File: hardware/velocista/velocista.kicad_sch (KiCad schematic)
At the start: 15 parts, among them J1 XT30, J2 Cable_PAD, J3 Cable_PAD, J4 QTR8a, SW1 SW_Push, SW3 SW_SPDT, U1 TB6612FNG, U2 Mini360, U3 ESP32_DEVKITC

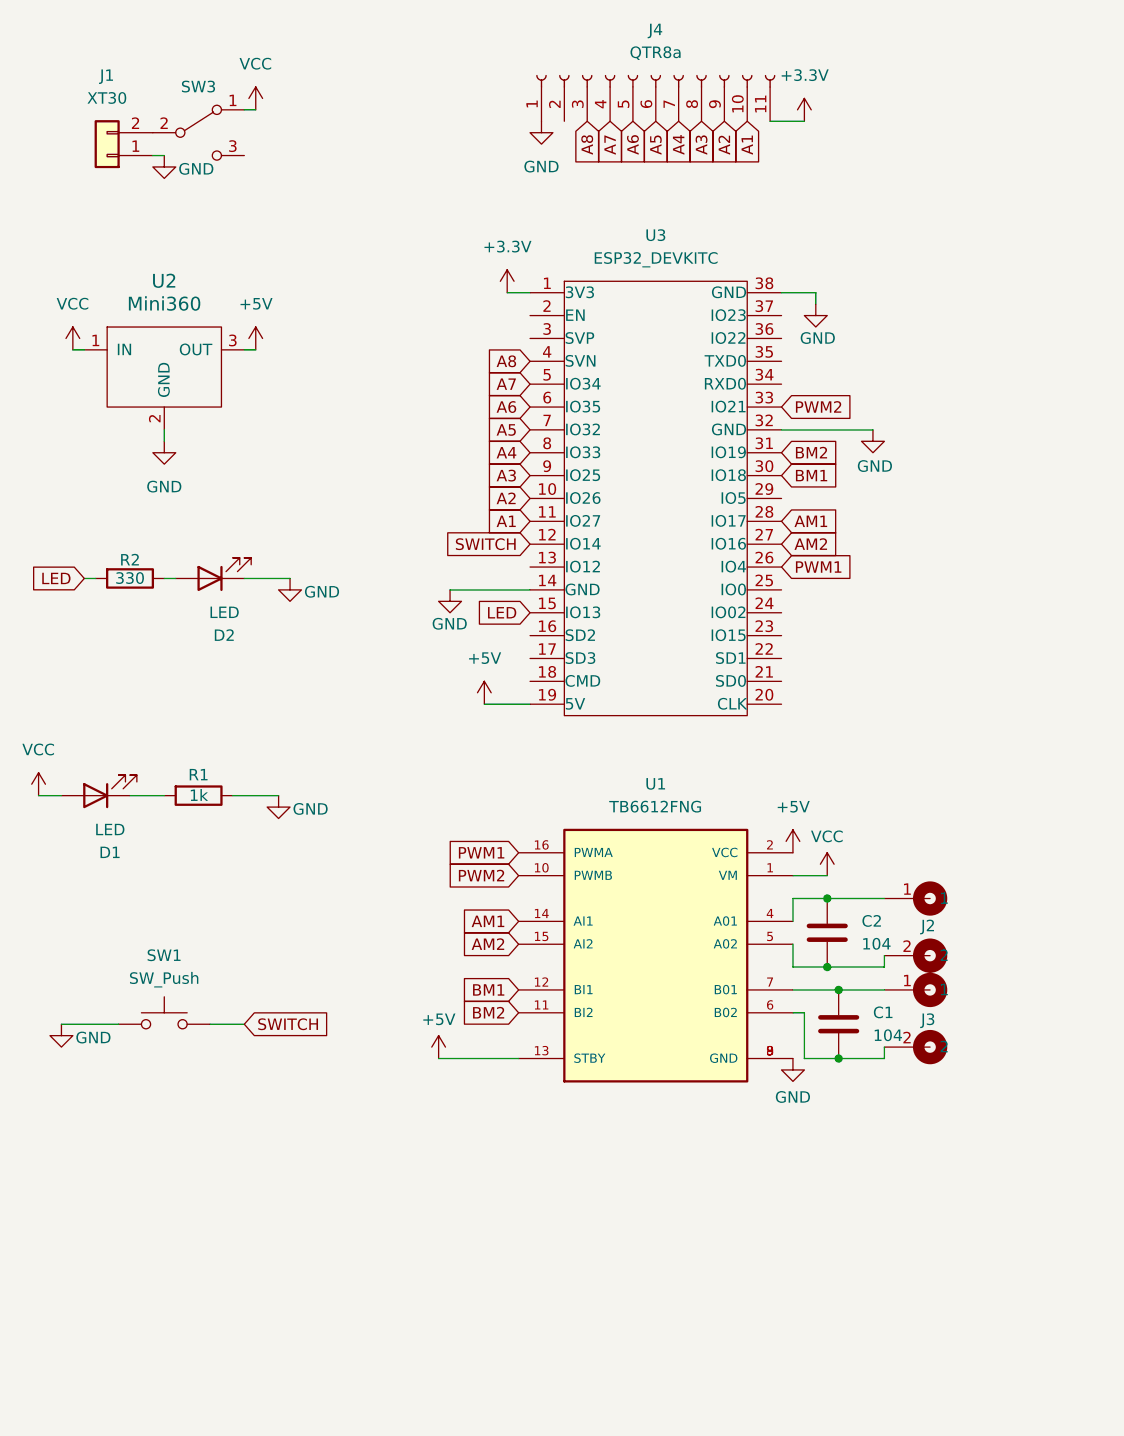
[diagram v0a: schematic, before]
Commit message: act pcb
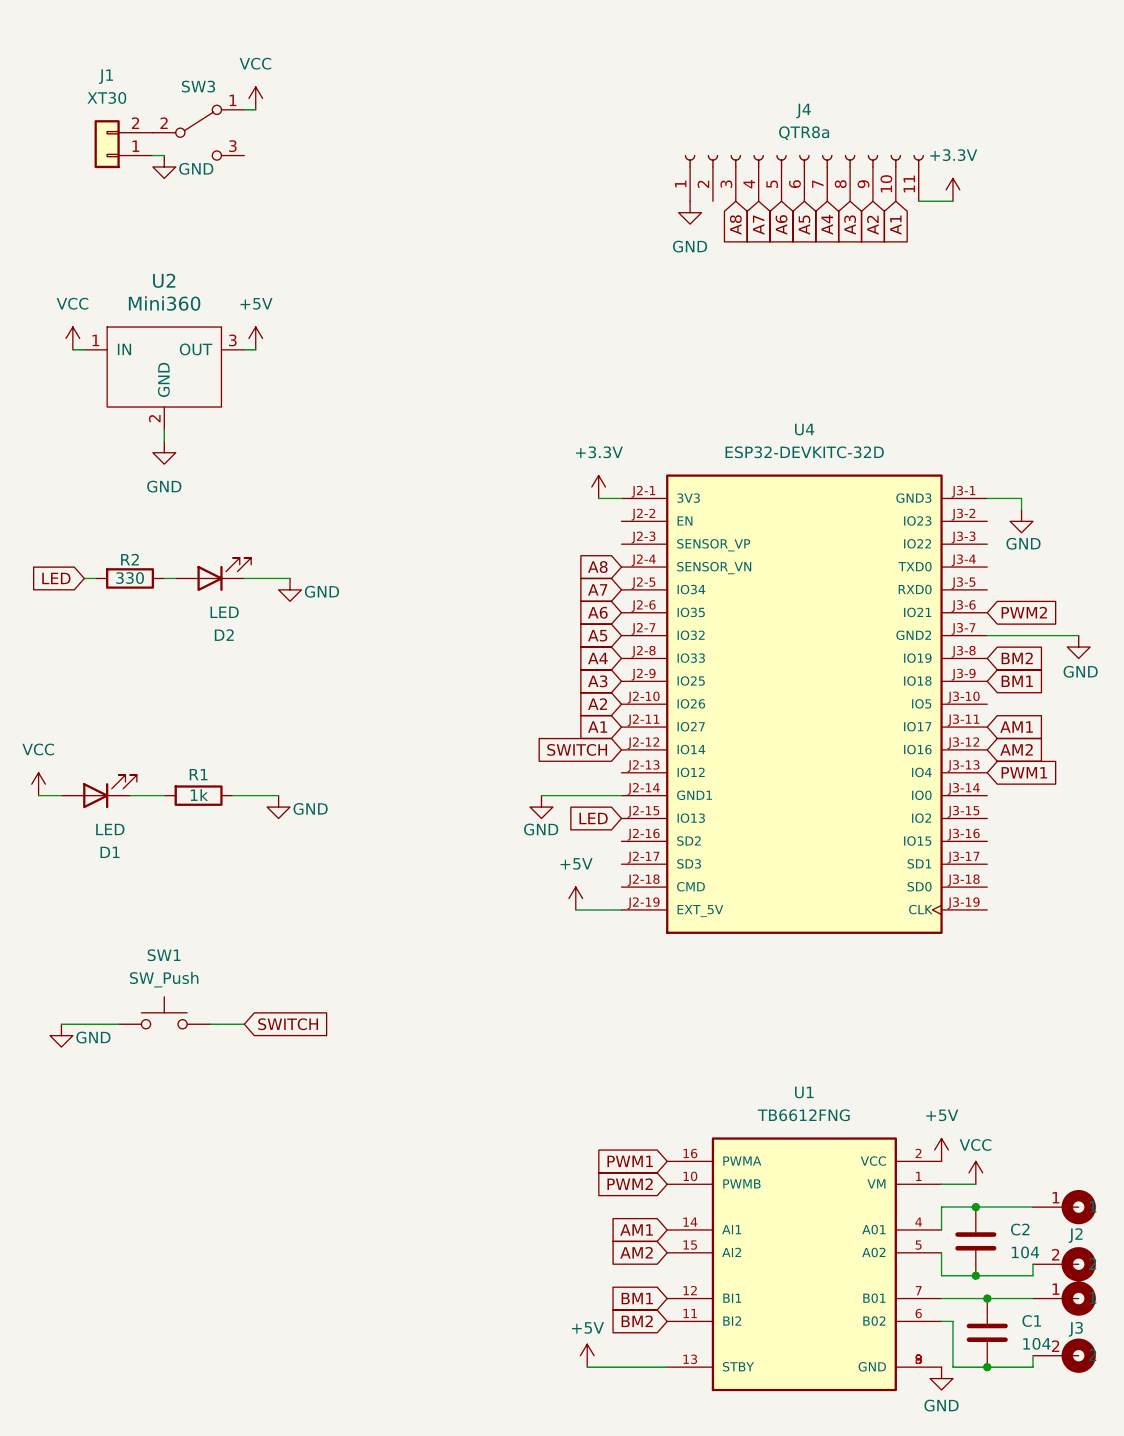
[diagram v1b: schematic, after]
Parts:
- removed U3: ESP32_DEVKITC, EESTN5:ESP32S, symbol EEESTN5:ESP32_DEVKITC
- added U4: ESP32-DEVKITC-32D, a:MODULE_ESP32-DEVKITC-32D, symbol ESP32-DEVKITC-32xd:ESP32-DEVKITC-32D
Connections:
- net +3.3V: now also U4.J2-1 (3V3)
- net +5V: now also U4.J2-19 (EXT_5V)
- net A1: now also U4.J2-11 (IO27)
- net A2: now also U4.J2-10 (IO26)
- net A3: now also U4.J2-9 (IO25)
- net A4: now also U4.J2-8 (IO33)
- net A5: now also U4.J2-7 (IO32)
- net A6: now also U4.J2-6 (IO35)
- net A7: now also U4.J2-5 (IO34)
- net A8: now also U4.J2-4 (SENSOR_VN)
- net AM1: now also U4.J3-11 (IO17)
- net AM2: now also U4.J3-12 (IO16)
- net BM1: now also U4.J3-9 (IO18)
- net BM2: now also U4.J3-8 (IO19)
- net GND: now also U4.J2-14 (GND1), U4.J3-1 (GND3), U4.J3-7 (GND2)
- net LED: now also U4.J2-15 (IO13)
- net PWM1: now also U4.J3-13 (IO4)
- net PWM2: now also U4.J3-6 (IO21)
- net SWITCH: now also U4.J2-12 (IO14)
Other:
- moved on the sheet: C1, C2, J2, J3, J4, U1
